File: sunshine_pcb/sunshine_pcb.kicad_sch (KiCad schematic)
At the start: 56 parts, among them J1 PWRIN, J2 Conn_01x04, J3 PWROUT, J5 VerticalUSB, Q1 AO3400A, SW1 SW_SPST, U1 ESP32-S3-WROOM-1, U2 SPX1117M3, U3 LIS3MDL, U4 ADXL375, U8 USBLC6-2P6

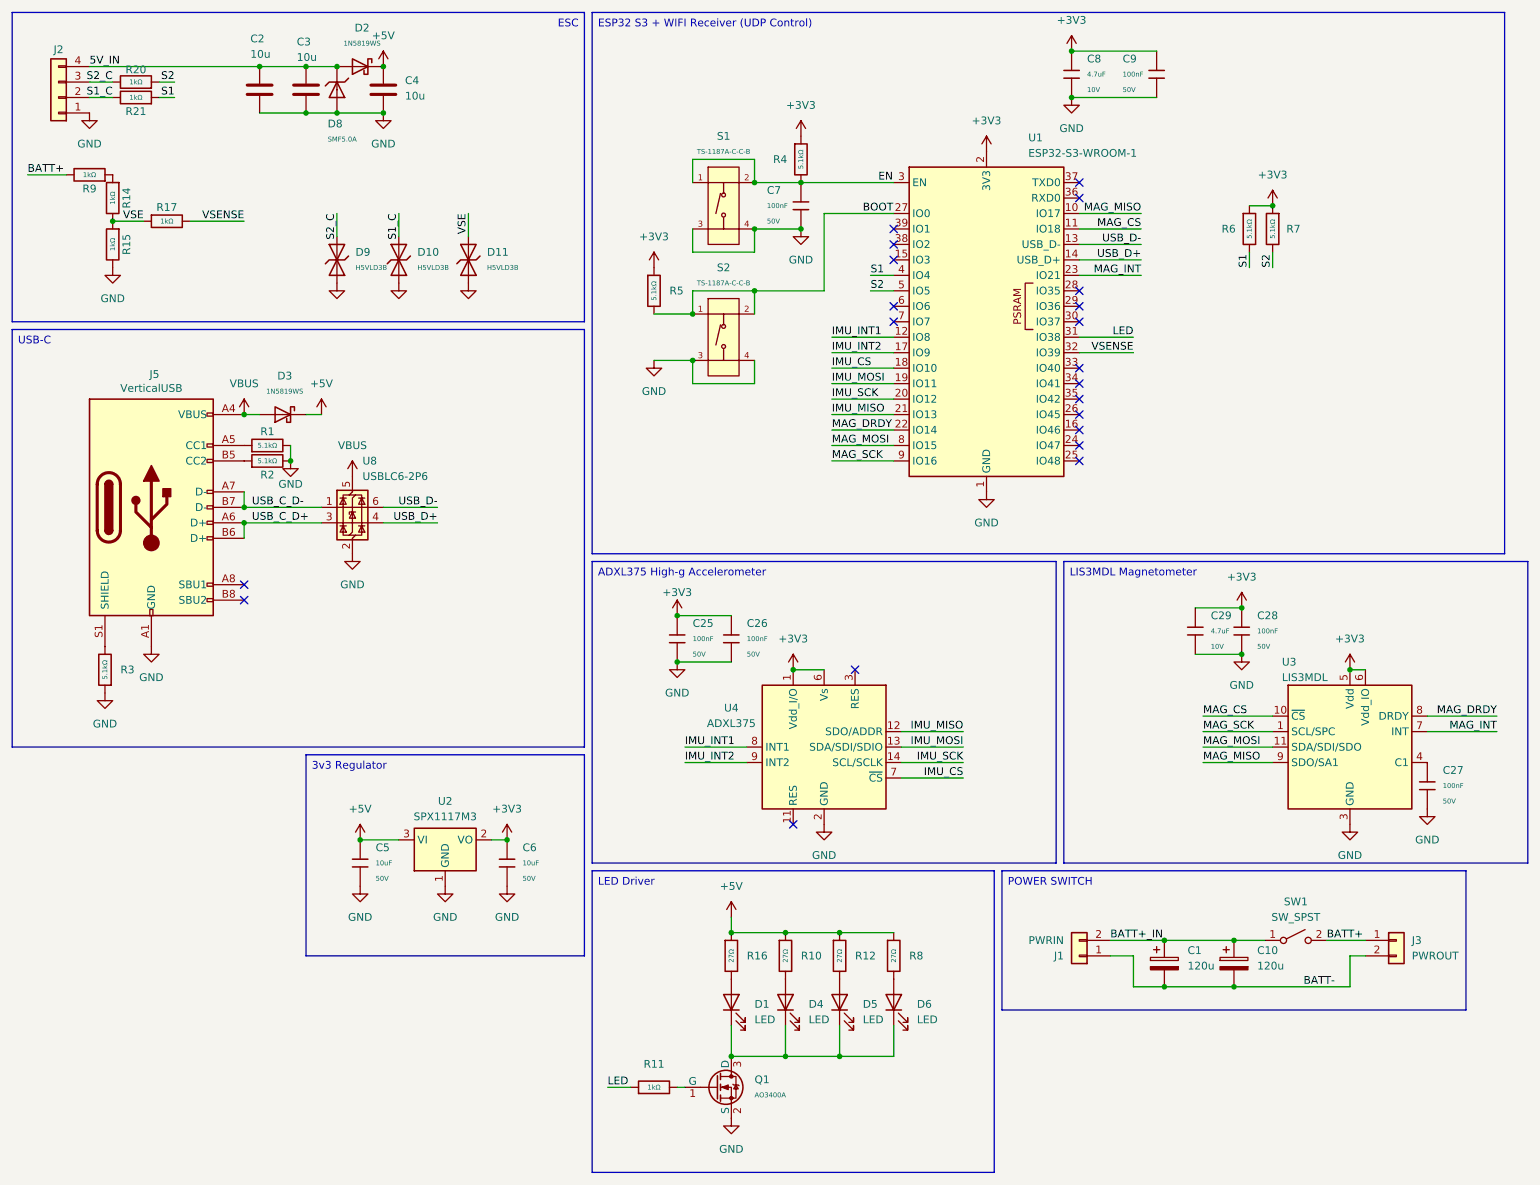
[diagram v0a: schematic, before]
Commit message: Re-layout PCB
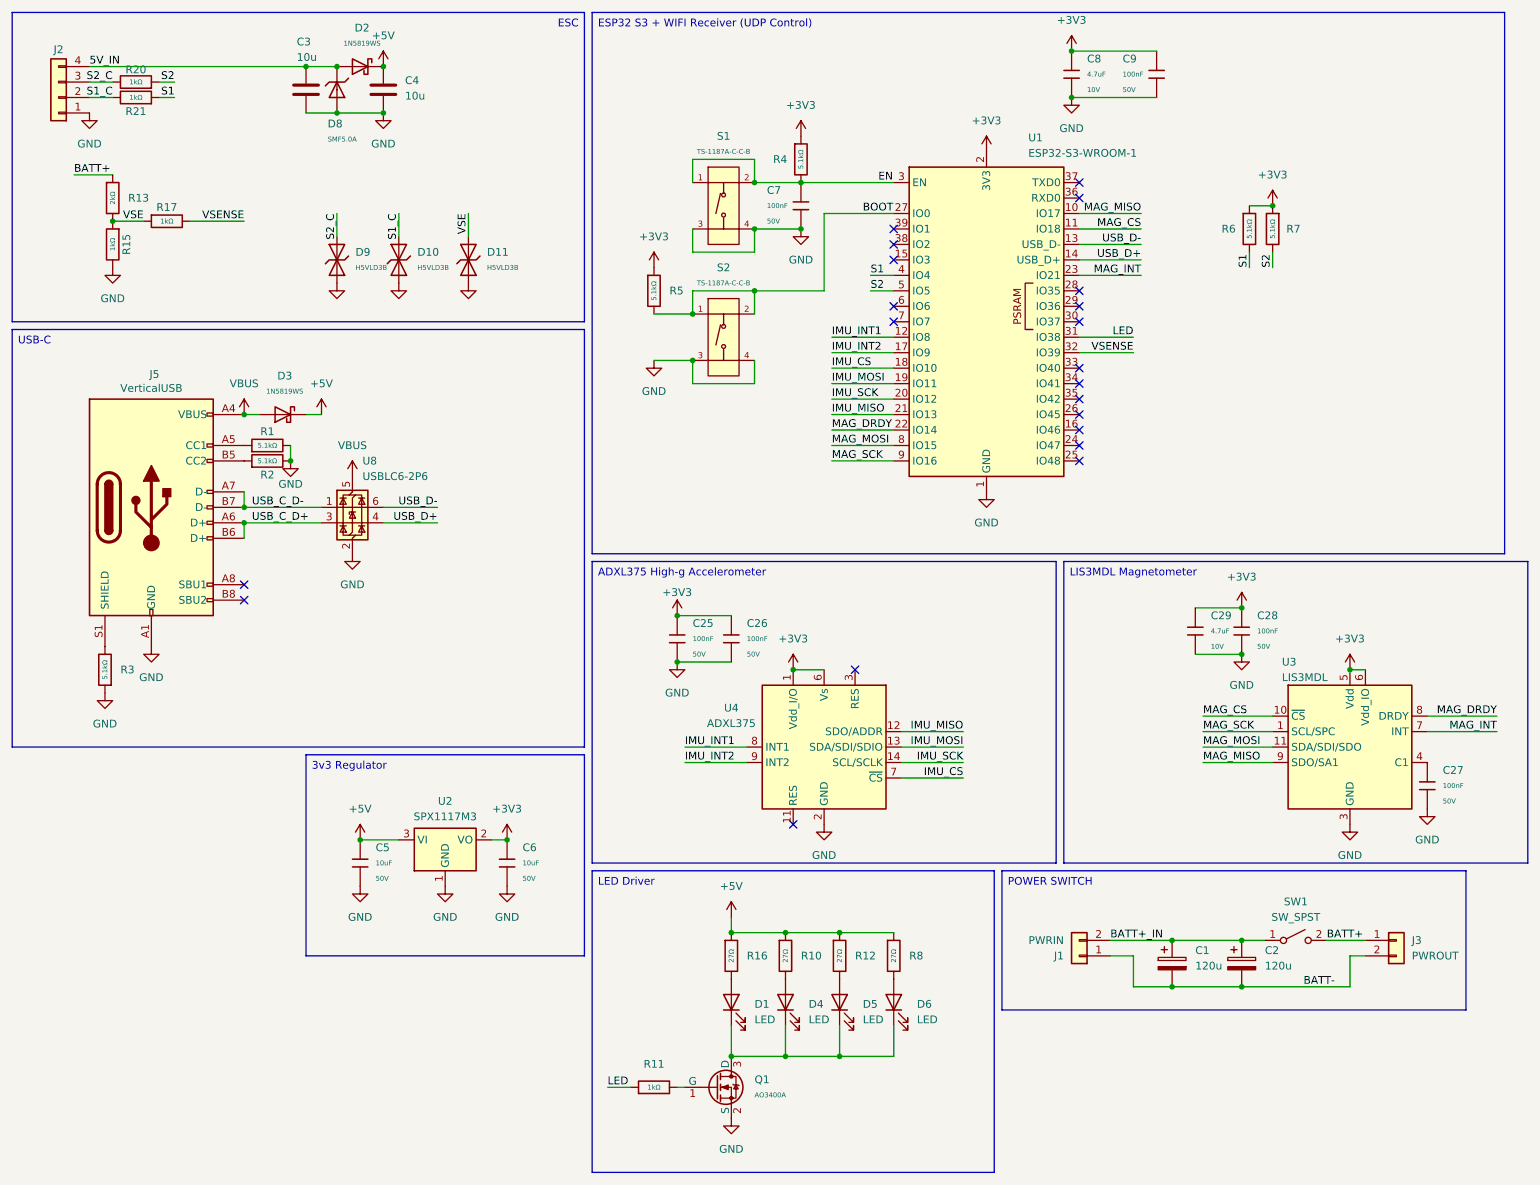
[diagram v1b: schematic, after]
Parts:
- removed C10: 120u, Capacitor_THT:CP_Radial_D6.3mm_P2.50mm, symbol Device:C_Polarized
- removed C2: 10u, Capacitor_SMD:C_1210_3225Metric, symbol Device:C
- removed R14, R9: 1kΩ, PCM_JLCPCB:R_0402, symbol PCM_JLCPCB-Resistors:0402,1kΩ
- added C2: 120u, Capacitor_THT:CP_Radial_D6.3mm_P2.50mm, symbol Device:C_Polarized
- added R13: 2kΩ, PCM_JLCPCB:R_0402, symbol PCM_JLCPCB-Resistors:0402,2kΩ
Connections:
- net BATT+: now also R13.1
- net BATT+_IN: now also C2.1
- net BATT-: now also C2.2
- net VSE: now also R13.2
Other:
- moved on the sheet: C1
